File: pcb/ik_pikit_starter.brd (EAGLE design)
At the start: 51.8 x 21.6 mm, 30 parts, among them U1 QRE1113, U2 MCP9700SMD

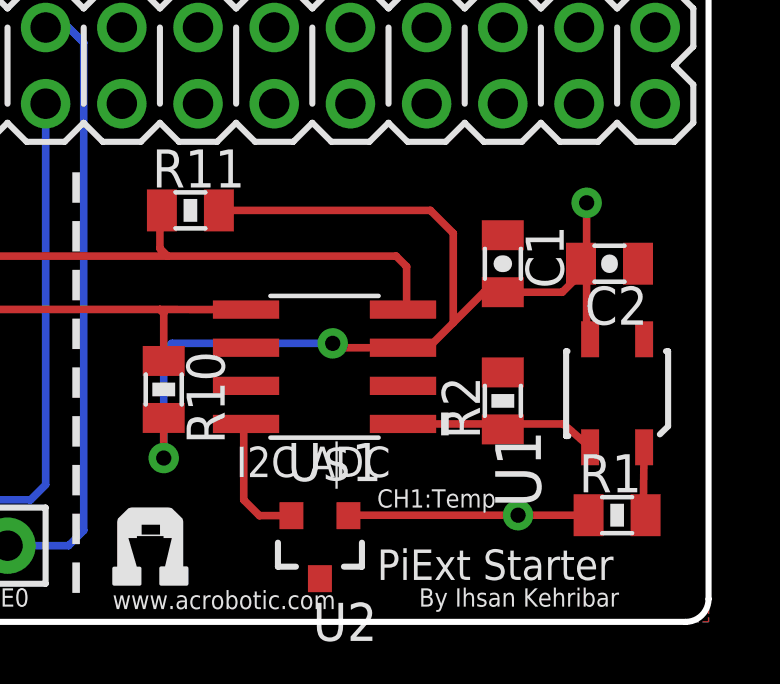
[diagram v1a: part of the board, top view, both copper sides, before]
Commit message: adding values
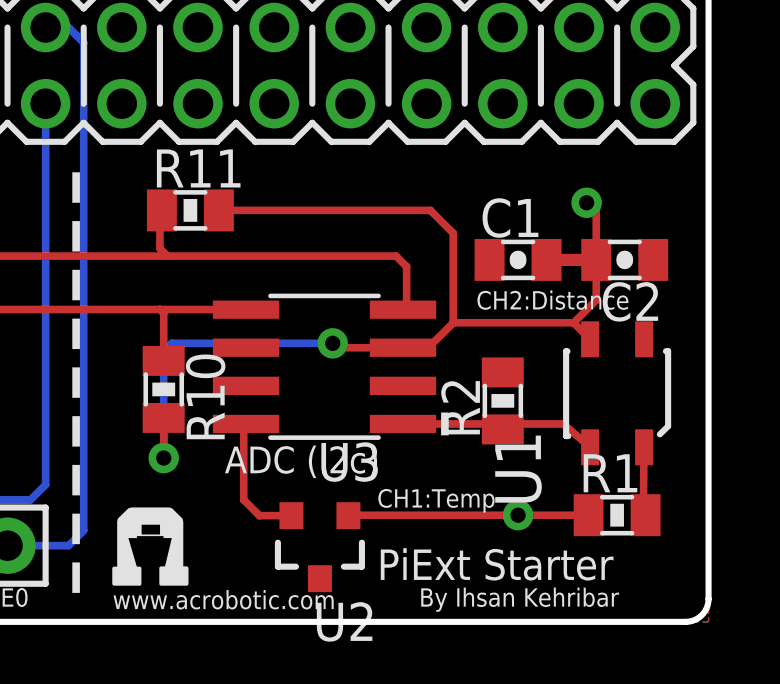
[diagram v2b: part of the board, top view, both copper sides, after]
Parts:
- C1, C2: value (none) -> 0.1uF
- LED1, LED2, LED3, LED4, LED5, LED6: value (none) -> BLUE
- R1: value (none) -> 100
- R10, R11, R3: value (none) -> 10K
- R2: value (none) -> 220
- R4, R5, R6, R7, R8, R9: value (none) -> 1K
- moved C1 0.52 mm to (45.5, 12.1), turned to 0 degrees
- moved C2 0.52 mm to (49.0, 12.1)
- renumbered U$1 to U3
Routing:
- net 3V3: track 46.4 -> 47.0 mm
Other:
- board text added: "ADC (i2c)"
- board text added: "CH2:Distance"
- board text removed: "I2C ADC"
